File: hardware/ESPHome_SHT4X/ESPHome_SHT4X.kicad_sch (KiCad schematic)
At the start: 15 parts, among them SW2 SW_Push, SW3 SW_Push, U1 ESP32-C6-WROOM-1-N8

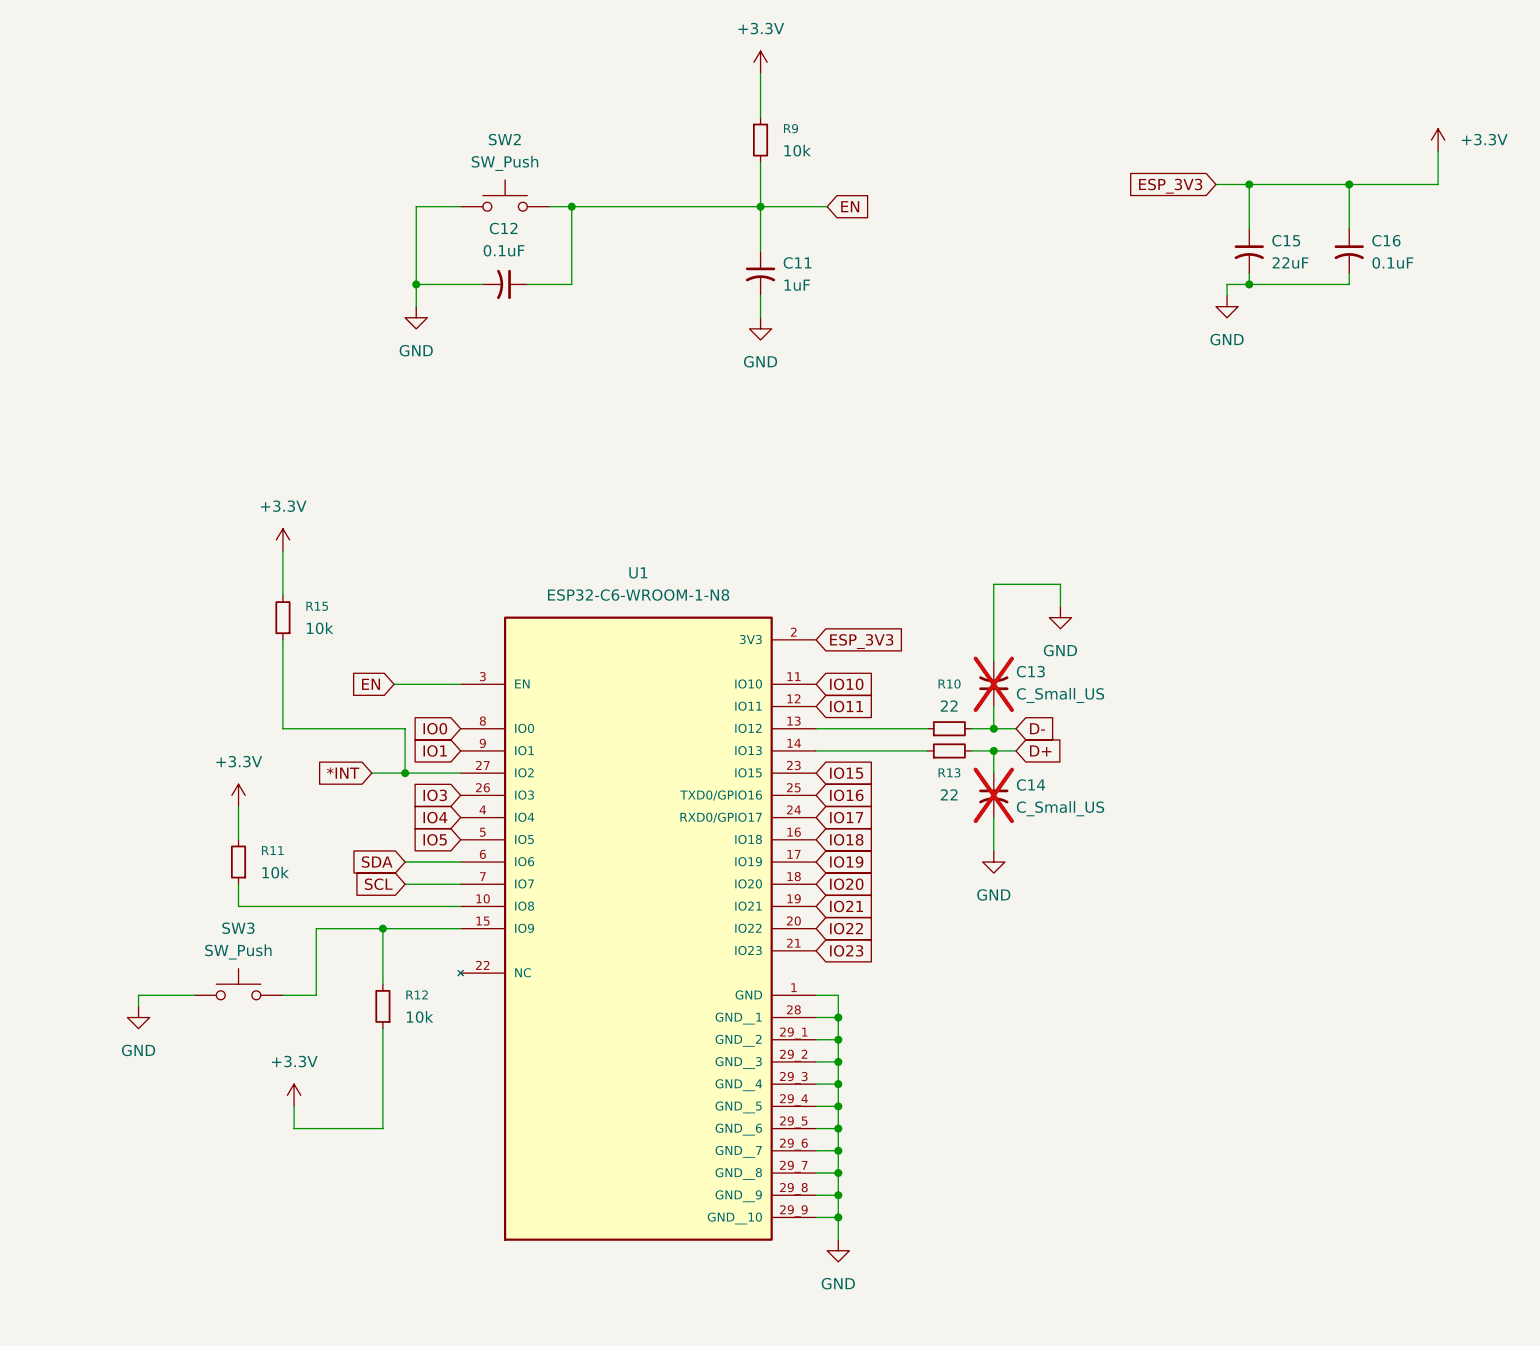
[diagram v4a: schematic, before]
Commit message: Working
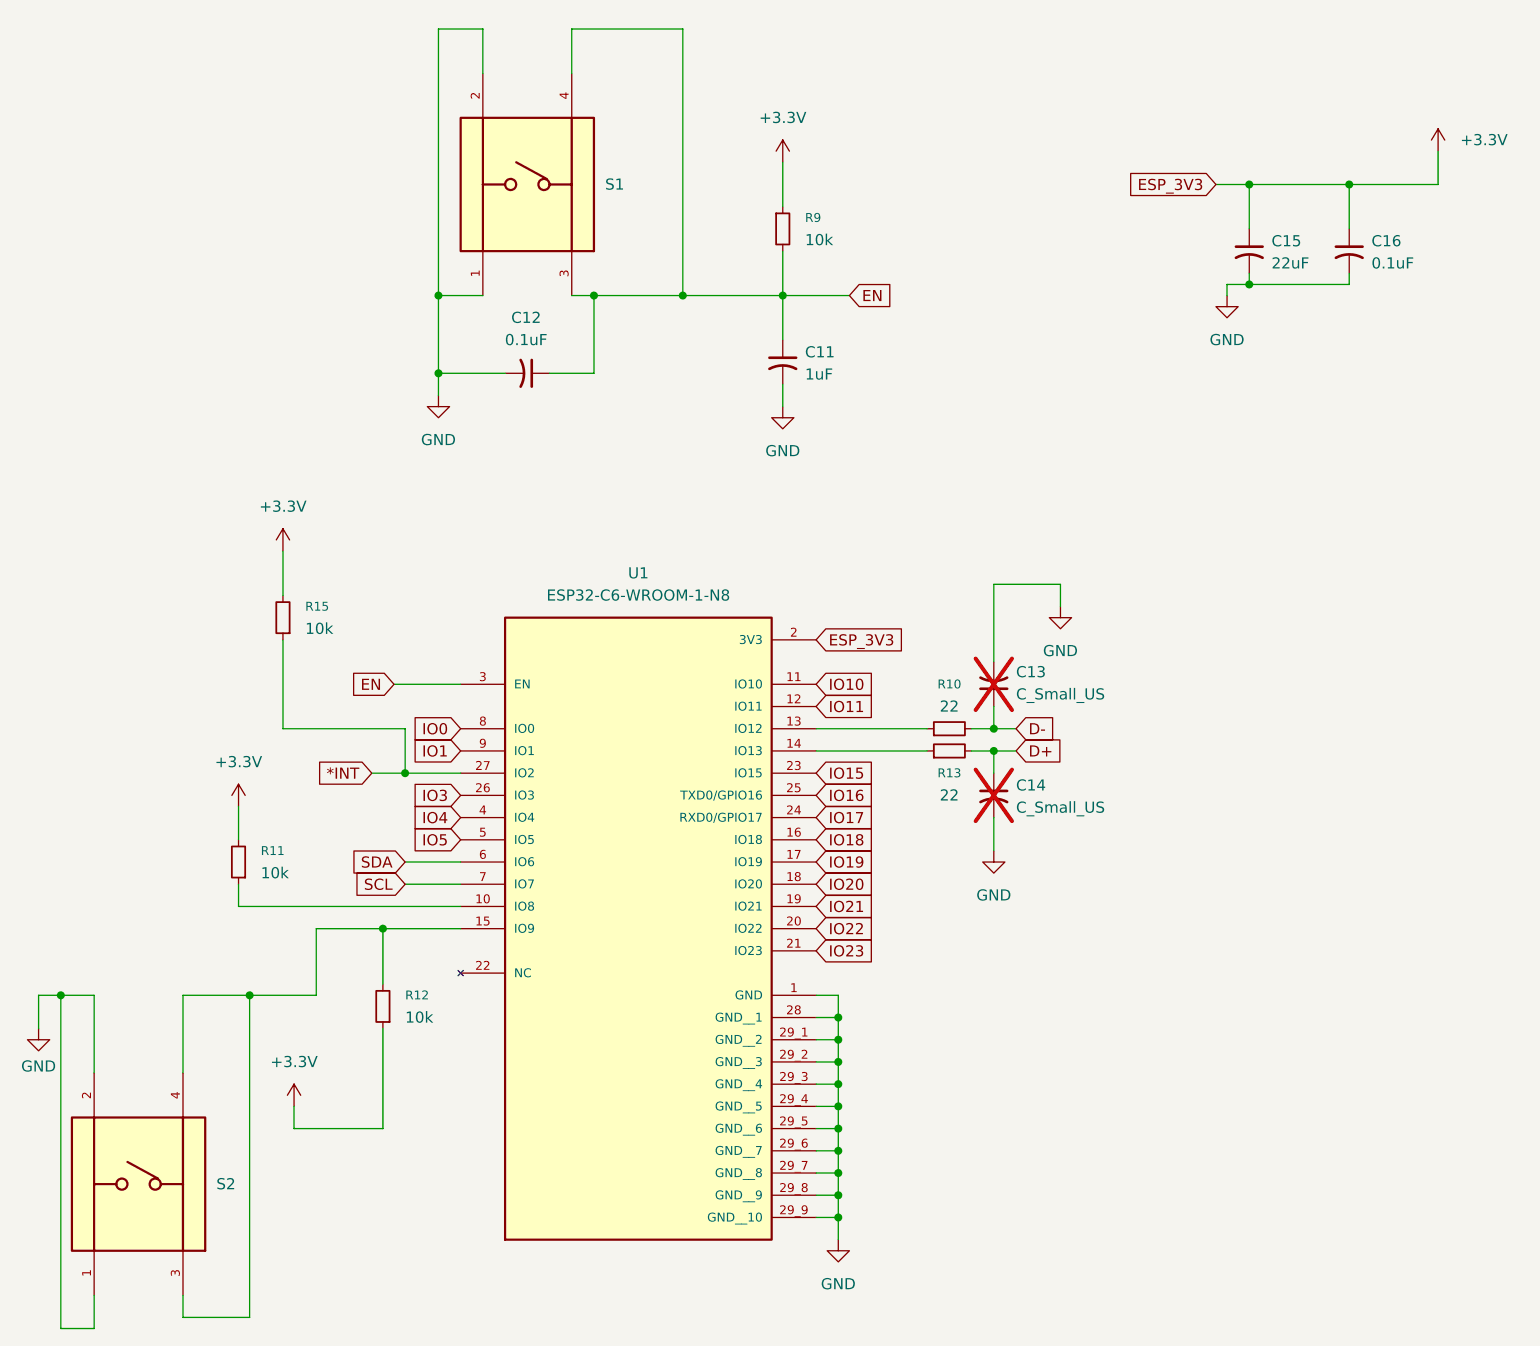
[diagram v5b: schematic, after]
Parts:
- removed SW2, SW3: SW_Push, Library:SW_TS02-66-43-BK-100-SCR-D, symbol Switch:SW_Push
- added S1, S2: TS02-66-43-BK-100-SCR-D, Library:SW_TS02-66-43-BK-100-SCR-D, symbol local:TS02-66-43-BK-100-SCR-D
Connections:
- net EN: now also S1.3, S1.4
- net GND: now also S1.1, S1.2, S2.1, S2.2
- net at R12.2, U1.15 (IO9): now also S2.3, S2.4
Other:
- moved on the sheet: C11, C12, R9

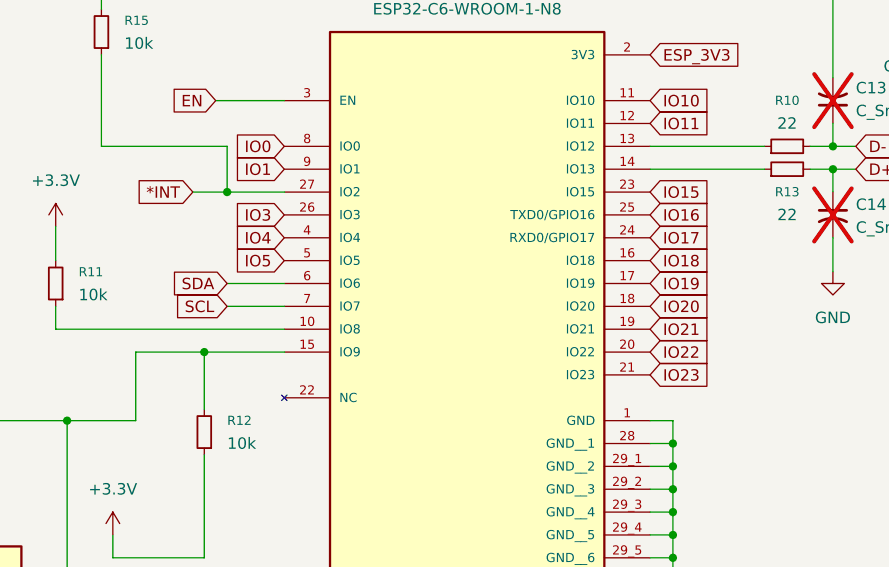
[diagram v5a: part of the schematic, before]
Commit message: Working
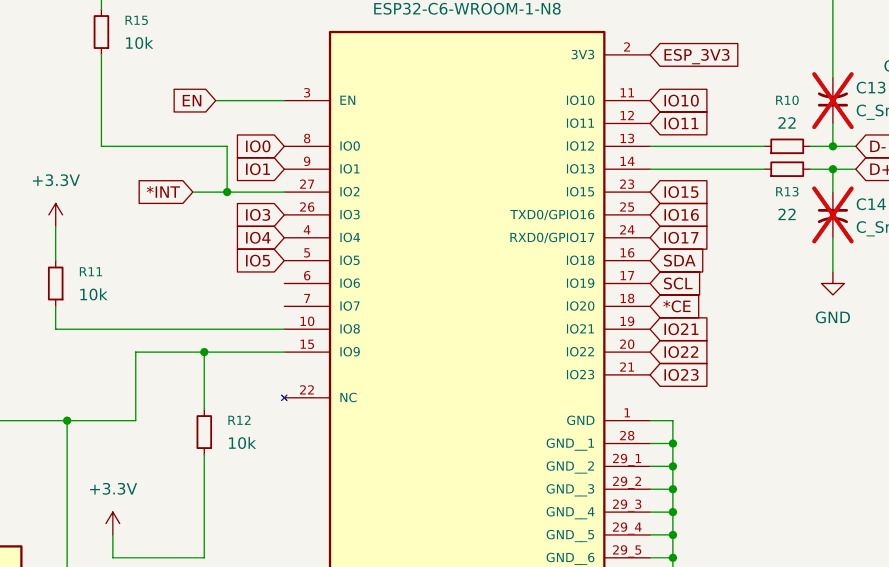
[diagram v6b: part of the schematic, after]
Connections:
- net IO18 is gone; now on net SDA: U1.16 (IO18)
- net IO19 is gone; now on net SCL: U1.17 (IO19)
- net SCL: no longer U1.7 (IO7)
- net SDA: no longer U1.6 (IO6)
- net IO20 renamed *CE

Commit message: Working
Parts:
- C16: footprint Capacitor_SMD:C_0201_0603Metric_Pad0.64x0.40mm_HandSolder -> Capacitor_SMD:C_0201_0603Metric
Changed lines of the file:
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@@
 			)
 		)
-		(property "Footprint" "Capacitor_SMD:C_0201_0603Metric_Pad0.64x0.40mm_HandSolder"
+		(property "Footprint" "Capacitor_SMD:C_0201_0603Metric"
 			(at 167.64 54.61 0)
 			(hide yes)
